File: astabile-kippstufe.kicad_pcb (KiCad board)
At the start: 2 copper layers, 57 x 32 mm, 16 parts, among them X1 +UB, X2 0V

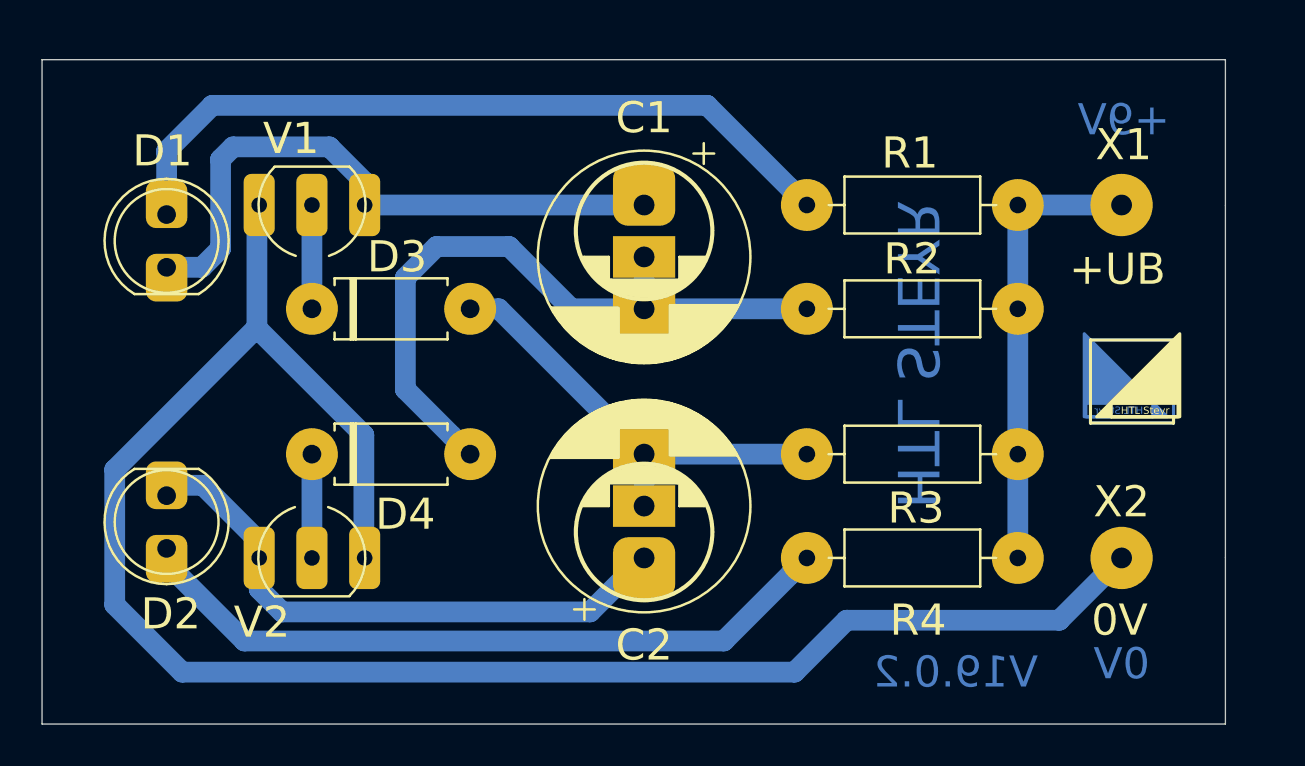
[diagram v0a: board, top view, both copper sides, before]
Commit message: Montagelöcher
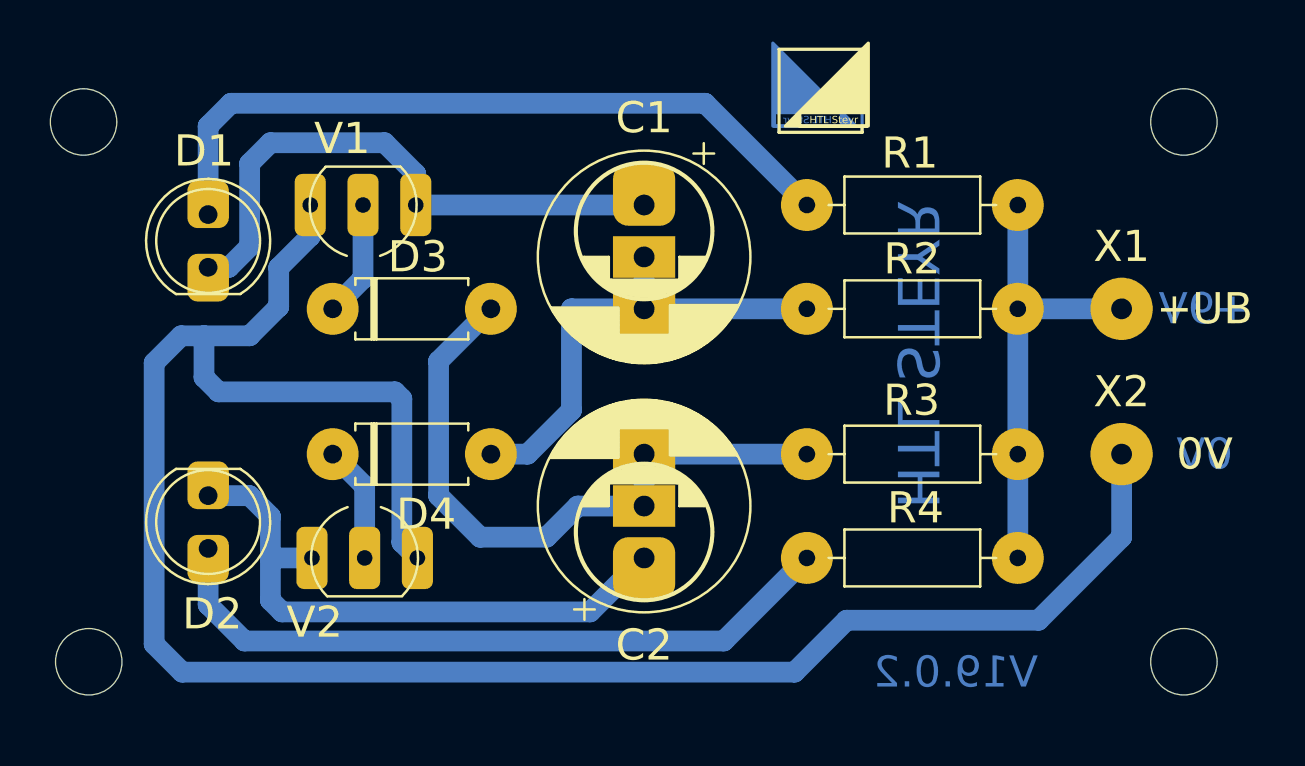
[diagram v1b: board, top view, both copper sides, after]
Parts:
- added H1: MountingHole, MountingHole:MountingHole_3.2mm_M3, F.Cu at (178.0, 71.0)
- added H2: MountingHole, MountingHole:MountingHole_3.2mm_M3, F.Cu at (178.0, 97.0)
- added H3: MountingHole, MountingHole:MountingHole_3.2mm_M3, F.Cu at (125.0, 71.0)
- added H4: MountingHole, MountingHole:MountingHole_3.2mm_M3, F.Cu at (125.2, 97.0)
- moved Logo1 20.5 mm to (160.5, 69.5)
- moved Logo2 20.5 mm to (160.5, 69.5)
- moved X1 5.00 mm to (175.0, 80.0)
- moved X2 5.00 mm to (175.0, 87.0)
- moved V2 2.54 mm to (136.0, 92.0)
- moved V1 2.46 mm to (141.0, 75.0)
- moved D1 2.00 mm to (131.0, 78.0)
- moved D2 2.00 mm to (131.0, 89.0)
- moved D3 1.00 mm to (137.0, 80.0)
- moved D4 1.00 mm to (137.0, 87.0)
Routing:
- net Net-(V1-Pad3): track 87.5 -> 100.0 mm
- net Net-(C2-Pad2): track 21.6 -> 31.7 mm
- net Net-(C1-Pad2): track 33.5 -> 23.5 mm
- net Net-(C1-Pad1): track 29.7 -> 27.9 mm
- net Net-(D1-Pad2): track 36.8 -> 35.6 mm
- net Net-(D2-Pad2): track 34.8 -> 33.9 mm
- net Net-(D4-Pad1): track 5.00 -> 5.64 mm
- net Net-(C2-Pad1): track 28.2 -> 28.8 mm
- net Net-(D3-Pad1): track 5.00 -> 5.60 mm
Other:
- board outline removed
